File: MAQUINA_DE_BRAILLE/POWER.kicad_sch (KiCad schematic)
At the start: 24 parts, among them J3 Screw_Terminal_01x02

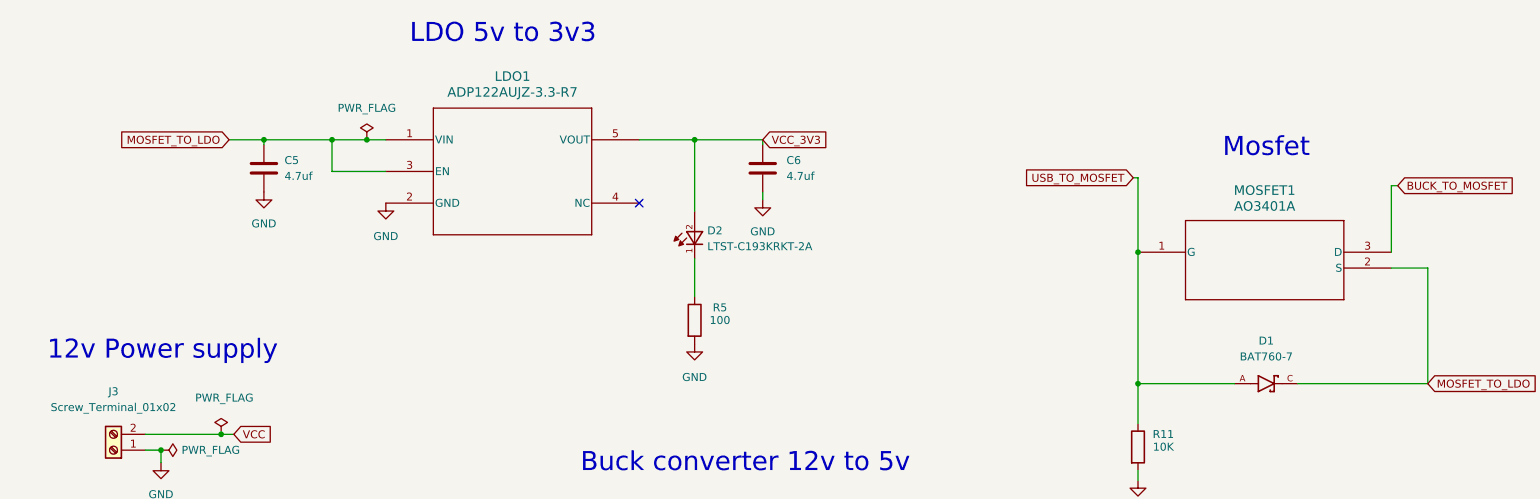
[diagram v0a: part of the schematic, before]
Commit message: LAST UPDATE
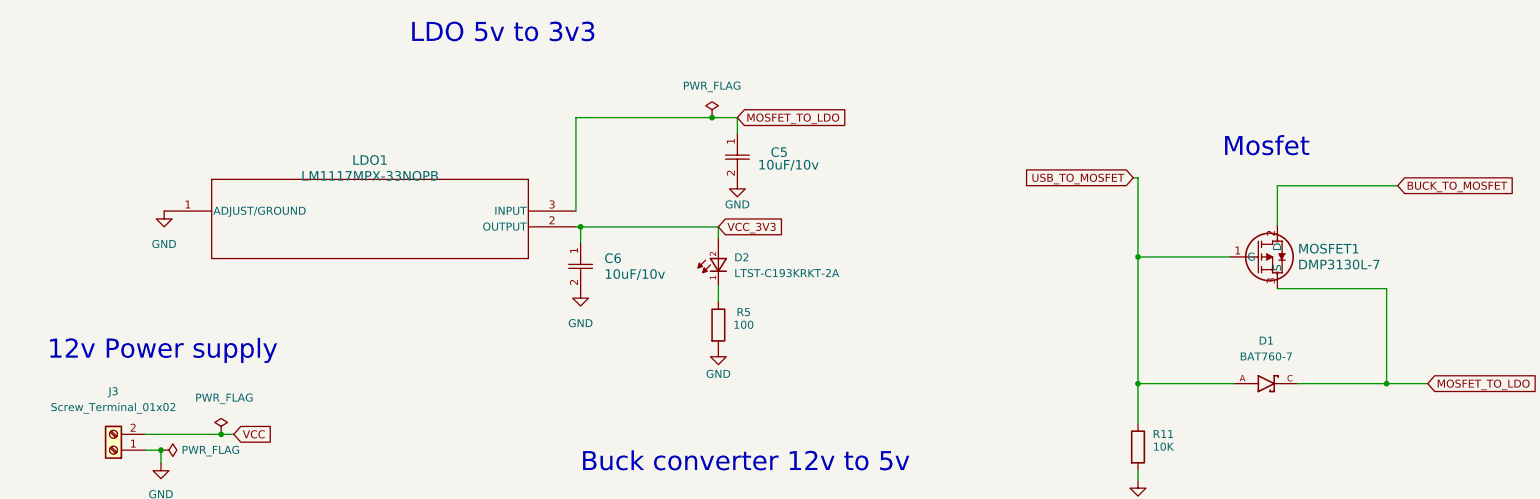
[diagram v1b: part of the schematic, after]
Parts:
- removed C5, C6: 4.7uf, Capacitor_SMD:C_0805_2012Metric_Pad1.18x1.45mm_HandSolder, symbol Device:C
- removed LDO1: ADP122AUJZ-3.3-R7, ADP122AUJZ_3_3_R7:UJ_5_ADI, symbol ADP122AUJZ-3.3-R7:ADP122AUJZ-3.3-R7
- removed MOSFET1: AO3401A, AO3401A:SOT-23-3L_AOS, symbol AO3401A:AO3401A
- added C5, C6: 10uF/10v, 293D106X9010A2TE3:CAP_293D-A_VSS, symbol 293D106X9010A2TE3:293D106X9010A2TE3
- added LDO1: LM1117MPX-33NOPB, LM1117:SOT223-318H_OSI, symbol LM1117:LM1117MPX-33NOPB
- added MOSFET1: DMP3130L-7, DMP3130L-7:SOT-23_DMP3130L_DIO, symbol DMP3130L-7:DMP3130L-7
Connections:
- net BUCK_TO_MOSFET: now also MOSFET1.2 (D)
- net GND: now also C5.2, C6.2, LDO1.1 (ADJUST/GROUND)
- net MOSFET_TO_LDO: now also C5.1, LDO1.3 (INPUT), MOSFET1.3 (S)
- net USB_TO_MOSFET: now also MOSFET1.1 (G)
- net VCC_3V3: now also C6.1, LDO1.2 (OUTPUT)
- no-connect marks 1 -> 0
